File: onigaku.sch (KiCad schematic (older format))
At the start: 364 parts, among them J1 MJ-4PP-9, J2 MJ-4PP-9, U1 Elite-C, U2 Elite-C

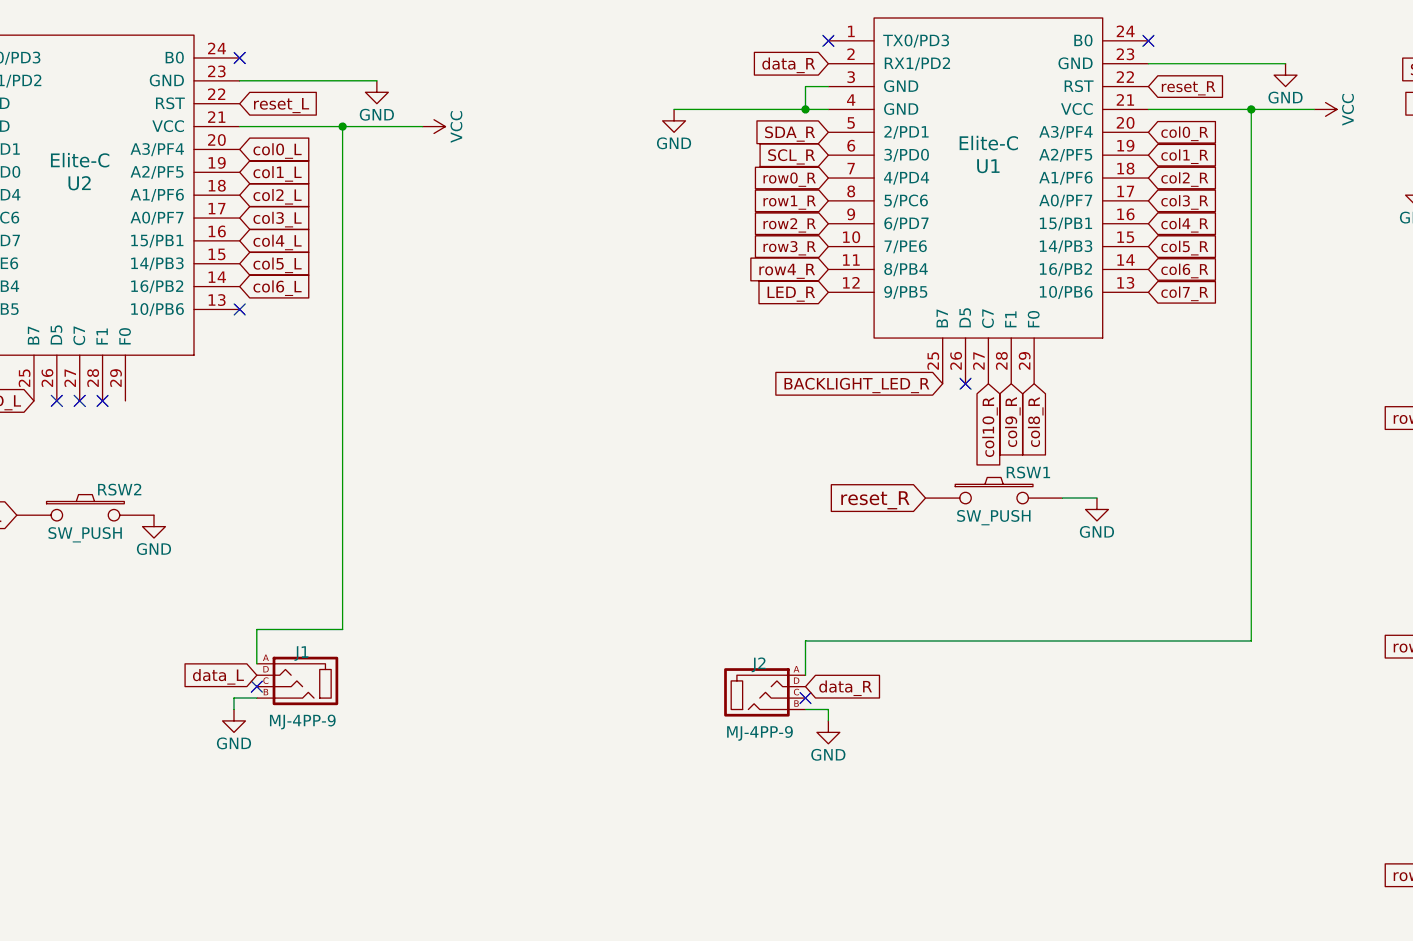
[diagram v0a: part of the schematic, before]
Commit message: wired up and still thinking
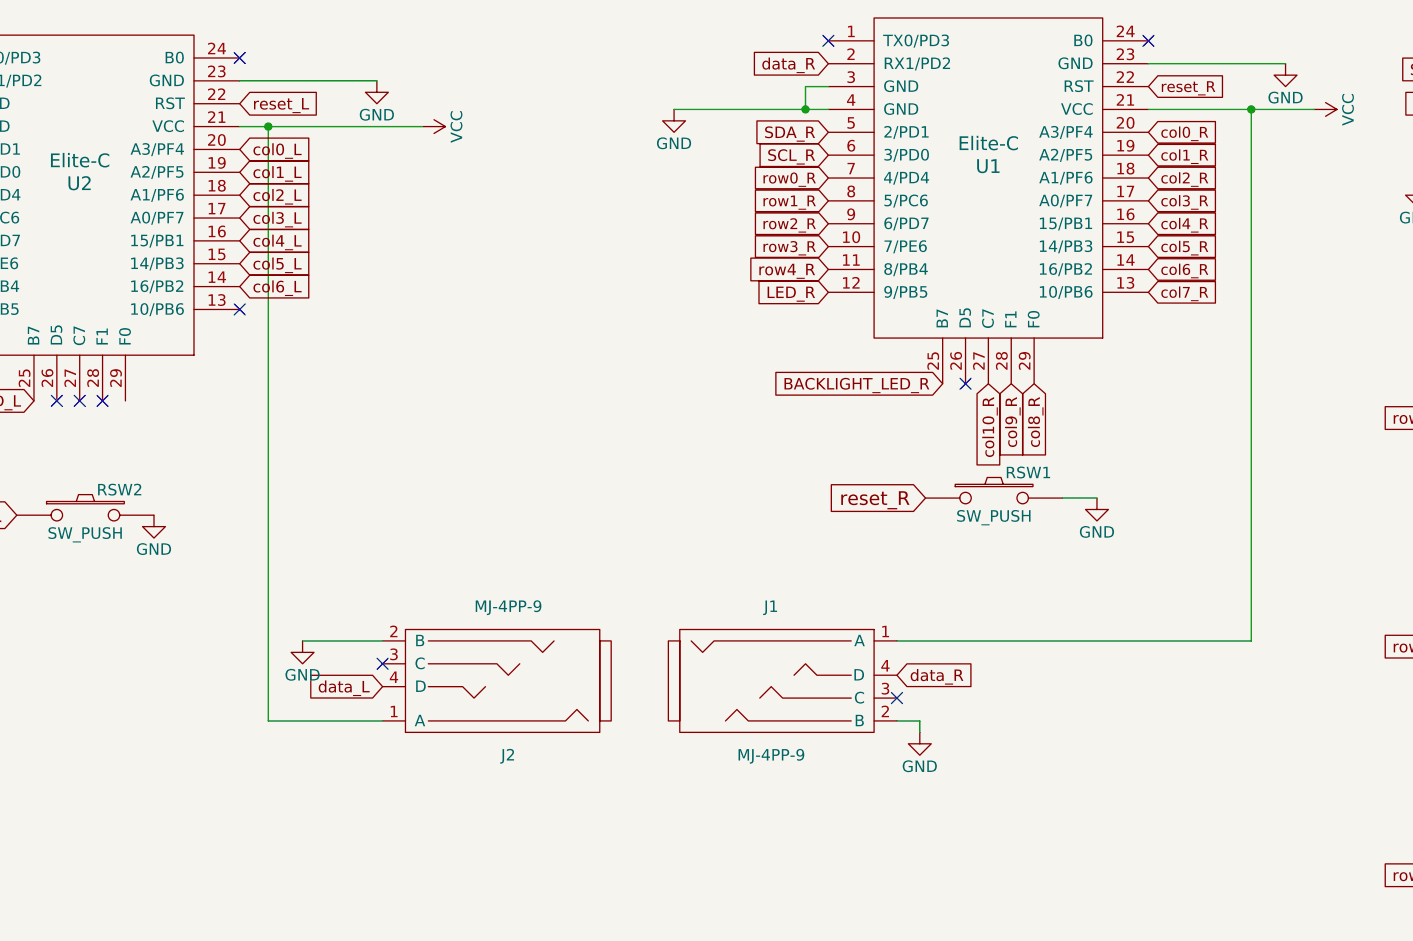
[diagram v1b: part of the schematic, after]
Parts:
- removed J1, J2: MJ-4PP-9, kbd:MJ-4PP-9_1side, symbol kbd:MJ-4PP-9
- added J1, J2: MJ-4PP-9, mj-4pp-9:MJ-4PP-9, symbol mj-4pp-9:MJ-4PP-9
- RSW1, RSW2: footprint kbd:ResetSW_1side -> Button_Switch_SMD:SW_SPST_TL3342
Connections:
- net GND: now also J1.2 (B), J2.2 (B)
- net VCC: now also J1.1 (A), J2.1 (A)
- net data_L: now also J2.4 (D)
- net data_R: now also J1.4 (D)
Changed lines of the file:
@@
 L power:GND #PWR015
 U 1 1 604F807D
-P 11325 4075
-F 0 "#PWR015" H 11325 3825 50  0001 C CNN
-F 1 "GND" H 11325 3925 50  0000 C CNN
-F 2 "" H 11325 4075 50  0001 C CNN
-F 3 "" H 11325 4075 50  0001 C CNN
-	1    11325 4075
-	-1   0    0    -1
+P 11625 3775
+F 0 "#PWR015" H 11625 3525 50  0001 C CNN
+F 1 "GND" H 11625 3625 50  0000 C CNN
+F 2 "" H 11625 3775 50  0001 C CNN
+F 3 "" H 11625 3775 50  0001 C CNN
+	1    11625 3775
+	1    0    0    -1
 $EndComp
-Wire Wire Line
-	11325 4075 11325 4025
 $Comp
 L kbd:SW_PUSH RSW2
@@
 F 0 "RSW2" H 10825 3335 50  0000 C CNN
 F 1 "SW_PUSH" H 10675 3145 50  0000 C CNN
-F 2 "kbd:ResetSW_1side" H 10675 3225 50  0001 C CNN
+F 2 "Button_Switch_SMD:SW_SPST_TL3342" H 10675 3225 50  0001 C CNN
 F 3 "" H 10675 3225 50  0000 C CNN
 	1    10675 3225
@@
 F 0 "RSW1" H 14800 3260 50  0000 C CNN
 F 1 "SW_PUSH" H 14650 3070 50  0000 C CNN
-F 2 "kbd:ResetSW_1side" H 14650 3150 50  0001 C CNN
+F 2 "Button_Switch_SMD:SW_SPST_TL3342" H 14650 3150 50  0001 C CNN
 F 3 "" H 14650 3150 50  0000 C CNN
 	1    14650 3150
@@
 Connection ~ 4350 5450
 Wire Wire Line
-	11425 4025 11325 4025
-Wire Wire Line
-	11425 3725 11425 3875
-Wire Wire Line
-	13825 4075 13925 4075
-Wire Wire Line
-	13825 3775 13825 3925
+	14225 4125 14325 4125
 Wire Wire Line
 	3575 8250 3775 8250
@@
 	5150 8250 5300 8250
 $Comp
-L kbd:MJ-4PP-9 J1
-U 1 1 5ACD605D
-P 11625 3975
-F 0 "J1" H 11625 4125 50  0000 C CNN
-F 1 "MJ-4PP-9" H 11625 3825 50  0000 C CNN
-F 2 "kbd:MJ-4PP-9_1side" H 11900 4150 50  0001 C CNN
-F 3 "" H 11900 4150 50  0001 C CNN
-	1    11625 3975
-	-1   0    0    -1
-$EndComp
-$Comp
 L kbd:YS-SK6812MINI-E LED33
 U 1 1 604F8029
@@
 $EndComp
 $Comp
-L kbd:MJ-4PP-9 J2
-U 1 1 604F805B
-P 13625 4025
-F 0 "J2" H 13625 4175 50  0000 C CNN
-F 1 "MJ-4PP-9" H 13625 3875 50  0000 C CNN
-F 2 "kbd:MJ-4PP-9_1side" H 13900 4200 50  0001 C CNN
-F 3 "" H 13900 4200 50  0001 C CNN
-	1    13625 4025
-	1    0    0    -1
-$EndComp
-$Comp
 L kbd:YS-SK6812MINI-E LED60
 U 1 1 60E11226
@@
 Text GLabel 13925 1250 0    50   Input ~ 0
 data_R
-Text GLabel 11425 3925 0    50   Input ~ 0
+Text GLabel 11975 3975 0    50   Input ~ 0
 data_L
 Text GLabel 9950 1325 0    50   Input ~ 0
@@
 NoConn ~ 13925 1150
 NoConn ~ 15325 1150
-Text GLabel 13825 3975 2    50   Input ~ 0
+Text GLabel 14225 3925 2    50   Input ~ 0
 data_R
-NoConn ~ 11425 3975
-NoConn ~ 13825 4025
+NoConn ~ 14225 4025
 $Comp
 L kbd:YS-SK6812MINI-E LED27
@@
 	15100 3150 14950 3150
 Wire Wire Line
-	11350 1525 11800 1525
-Wire Wire Line
-	11425 3725 11800 3725
-Wire Wire Line
-	11800 3725 11800 1525
-Connection ~ 11800 1525
+	11350 1525 11475 1525
+Connection ~ 11475 1525
 Wire Wire Line
-	11800 1525 12150 1525
+	11475 1525 12150 1525
 Wire Wire Line
 	16050 1450 15775 1450
@@
 	15775 1450 15775 3775
 Wire Wire Line
-	13825 3775 15775 3775
+	14225 3775 15775 3775
 Connection ~ 15775 1450
 Wire Wire Line
@@
 Connection ~ 13825 1450
 Wire Wire Line
-	13925 4125 13925 4075
+	14325 4175 14325 4125
 $Comp
 L power:PWR_FLAG #FLG0103
@@
 L power:GND #PWR0108
 U 1 1 6170662B
-P 13925 4125
-F 0 "#PWR0108" H 13925 3875 50  0001 C CNN
-F 1 "GND" H 13925 3975 50  0000 C CNN
-F 2 "" H 13925 4125 50  0001 C CNN
-F 3 "" H 13925 4125 50  0001 C CNN
-	1    13925 4125
+P 14325 4175
+F 0 "#PWR0108" H 14325 3925 50  0001 C CNN
+F 1 "GND" H 14325 4025 50  0000 C CNN
+F 2 "" H 14325 4175 50  0001 C CNN
+F 3 "" H 14325 4175 50  0001 C CNN
+	1    14325 4175
 	1    0    0    -1
 $EndComp
@@
 Wire Wire Line
 	24375 8500 25175 8500
+$Comp
+L mj-4pp-9:MJ-4PP-9 J2
+U 1 1 607CD277
+P 12525 3975
+F 0 "J2" H 12525 4275 50  0000 C CNN
+F 1 "MJ-4PP-9" H 12525 3625 50  0000 C CNN
+F 2 "mj-4pp-9:MJ-4PP-9" H 11925 3875 50  0001 C CNN
+F 3 "" H 11925 3875 50  0001 C CNN
+	1    12525 3975
+	-1   0    0    1
+$EndComp
+Wire Wire Line
+	11475 4125 11975 4125
+NoConn ~ 11975 3875
+Wire Wire Line
+	11475 1525 11475 4125
+Wire Wire Line
+	11625 3775 11975 3775
+$Comp
+L mj-4pp-9:MJ-4PP-9 J1
+U 1 1 60EC7D5C
+P 13675 3925
+F 0 "J1" H 13675 4225 50  0000 C CNN
+F 1 "MJ-4PP-9" H 13675 3575 50  0000 C CNN
+F 2 "mj-4pp-9:MJ-4PP-9" H 13075 3825 50  0001 C CNN
+F 3 "" H 13075 3825 50  0001 C CNN
+	1    13675 3925
+	1    0    0    -1
+$EndComp
 $EndSCHEMATC
